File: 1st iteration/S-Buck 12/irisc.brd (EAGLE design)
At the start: 44.1 x 33 mm, 14 parts, among them U1 LM2695MH

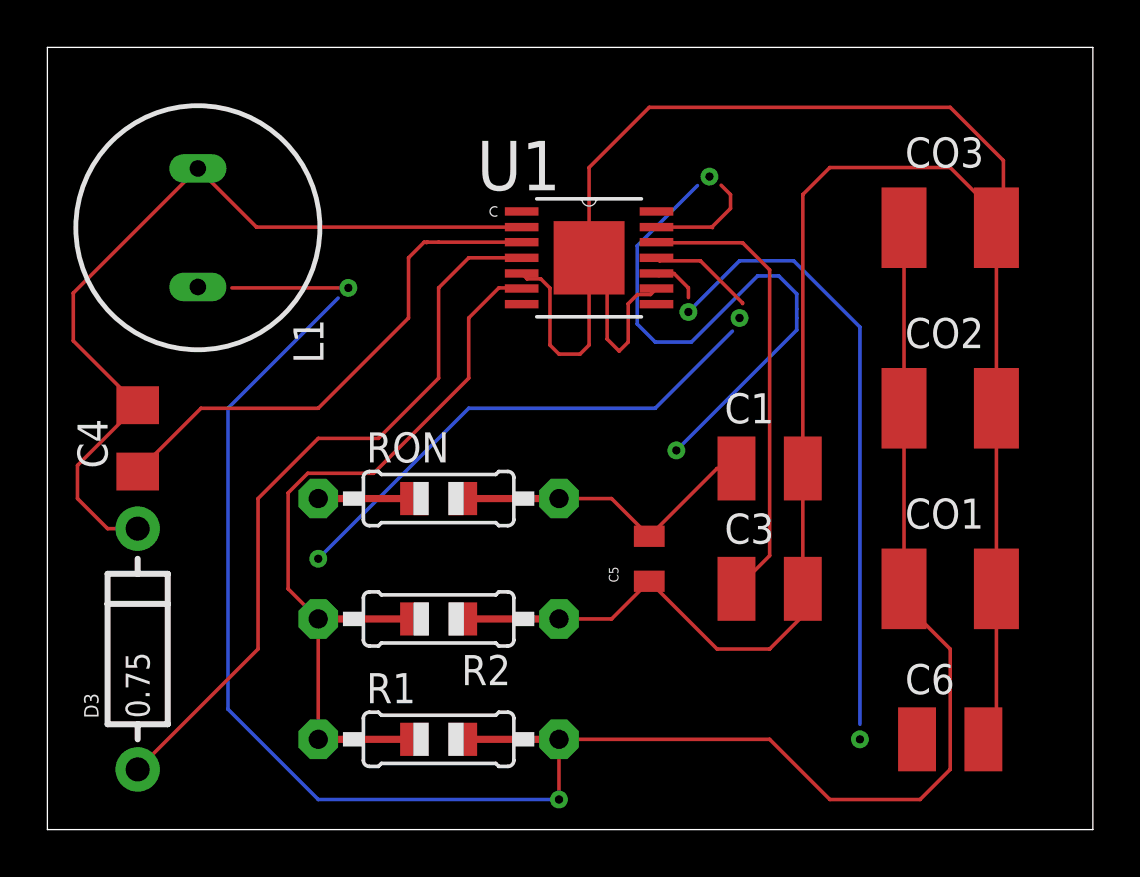
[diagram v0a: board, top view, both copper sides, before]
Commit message: Sabina Changes
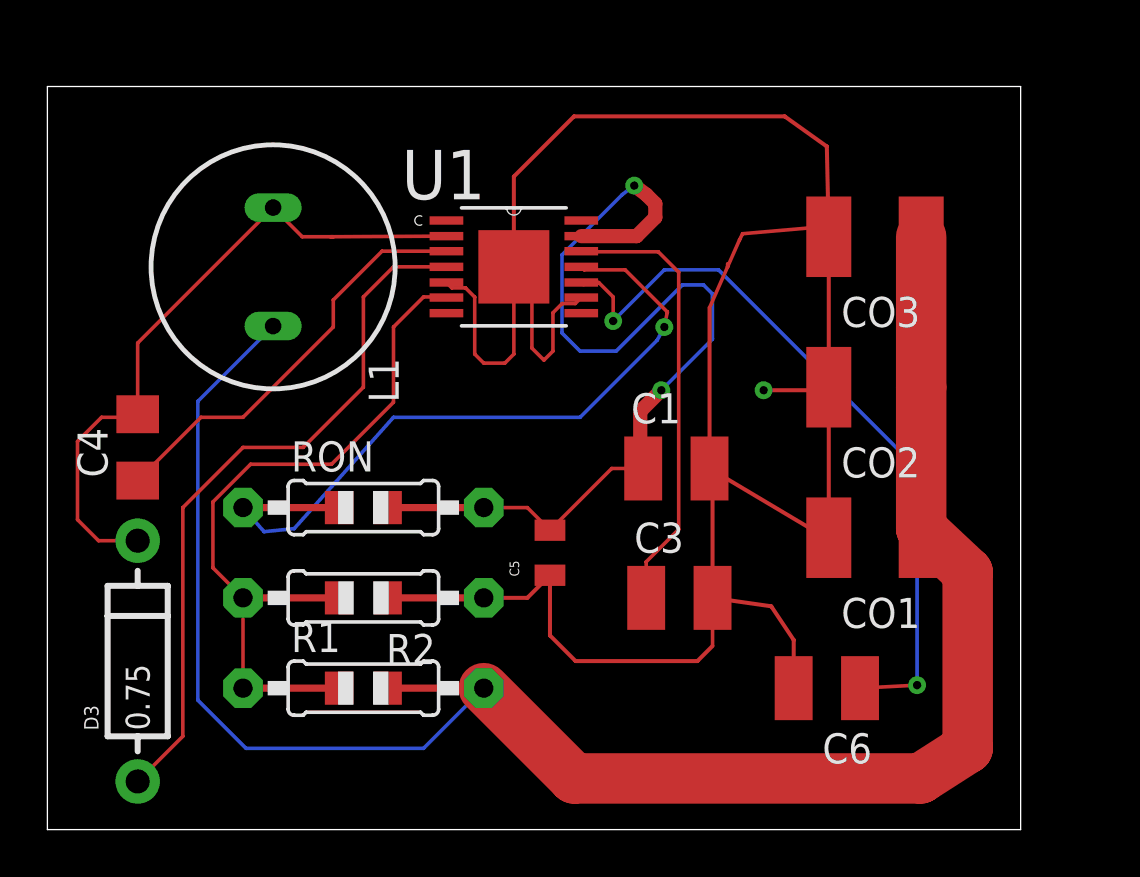
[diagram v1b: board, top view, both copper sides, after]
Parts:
- moved C6 5.64 mm to (32.9, 5.97), turned to 180 degrees
- moved C5 4.20 mm to (21.2, 11.7)
- moved C1 3.94 mm to (26.5, 15.2)
- moved CO1 3.84 mm to (34.9, 12.3), turned to 180 degrees
- moved R1 3.84 mm to (13.3, 5.97)
- moved C3 3.83 mm to (26.7, 9.78)
- moved L1 3.58 mm to (9.53, 23.7)
- moved CO2 3.30 mm to (34.9, 18.7), turned to 180 degrees
- moved R2 3.30 mm to (13.3, 9.78)
- moved CO3 3.20 mm to (34.9, 25.0), turned to 180 degrees
- moved RON 3.20 mm to (13.3, 13.6)
- moved U1 3.20 mm to (19.7, 23.7)
- moved D3 0.51 mm to (3.81, 7.11)
- moved C4 0.38 mm to (3.81, 16.1)
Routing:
- net N$1: track 34.8 -> 0.00 mm, vias 1 -> 0
- net 12V: track 44.3 -> 77.5 mm
- net N$128: track 2.15 -> 31.5 mm, vias 0 -> 2
- net N$6: track 26.1 -> 0.00 mm, vias 1 -> 0
- net N$7: track 24.1 -> 0.00 mm, vias 1 -> 0
- net VCC: track 14.0 -> 37.6 mm, vias 0 -> 2
- net N$127: track 4.45 -> 27.1 mm, vias 0 -> 1
- net N$3: track 21.5 -> 0.00 mm, vias 1 -> 0
- net N$126: track 36.0 -> 28.4 mm
- net GND: track 107.7 -> 101.8 mm, vias 0 -> 1
- net N$2: track 4.91 -> 0.00 mm, vias 1 -> 0
- net N$125: track 21.7 -> 17.7 mm
- net N$123: track 26.7 -> 22.8 mm
- net N$129: track 31.1 -> 29.9 mm
- net N$124: track 19.3 -> 18.8 mm
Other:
- board size 44.1 x 33 mm -> 41.1 x 31.4 mm
